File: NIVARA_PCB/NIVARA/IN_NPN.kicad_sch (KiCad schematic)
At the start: 0 parts

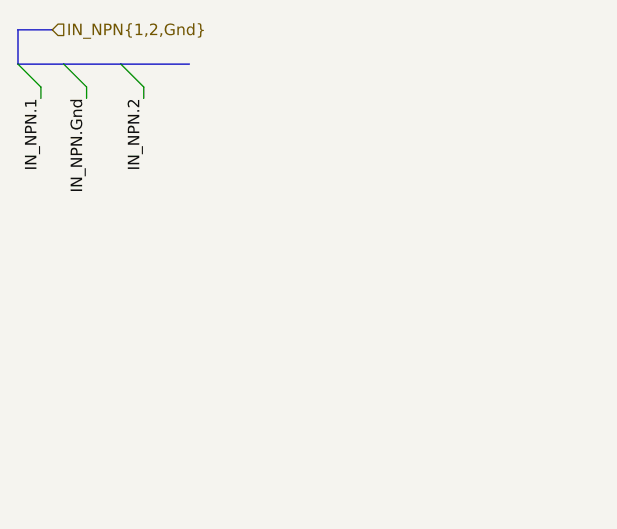
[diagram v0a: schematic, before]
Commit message: avance en diagramas
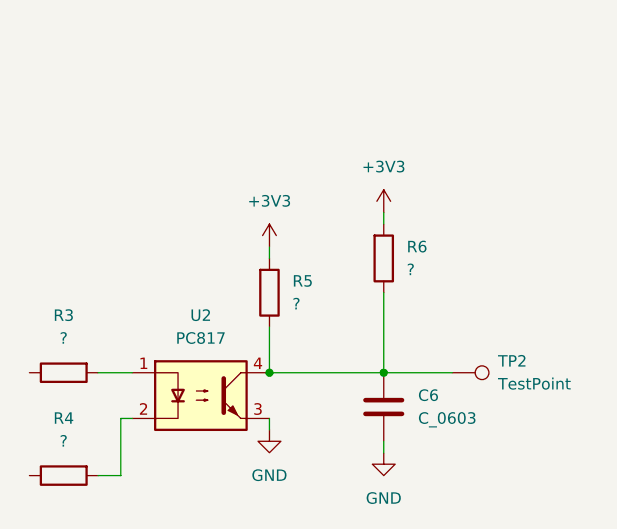
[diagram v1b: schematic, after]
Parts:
- added C6: C_0603, PCM_Capacitor_SMD_AKL:C_0603_1608Metric, symbol PCM_Capacitor_AKL:C_0603
- added R3, R4, R5, R6: ?, PCM_Resistor_SMD_AKL:R_0603_1608Metric, symbol PCM_Resistor_AKL:R_0603
- added TP2: TestPoint, symbol Connector:TestPoint
- added U2: PC817, PCM_Package_DIP_AKL:DIP-4_W7.62mm_SMDSocket_SmallPads, symbol Isolator:PC817
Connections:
- new net: C6.1, R5.2, R6.2, TP2.1, U2.4
- new net: R4.1, U2.2
- new net: R3.1, U2.1
- new net +3V3: R5.1, R6.1
- new net GND: C6.2, U2.3
